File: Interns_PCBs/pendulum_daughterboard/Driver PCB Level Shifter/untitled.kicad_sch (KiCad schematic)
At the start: 10 parts, among them U5 AMS1117-3.3, U6 SN74LVC2T45DCUR

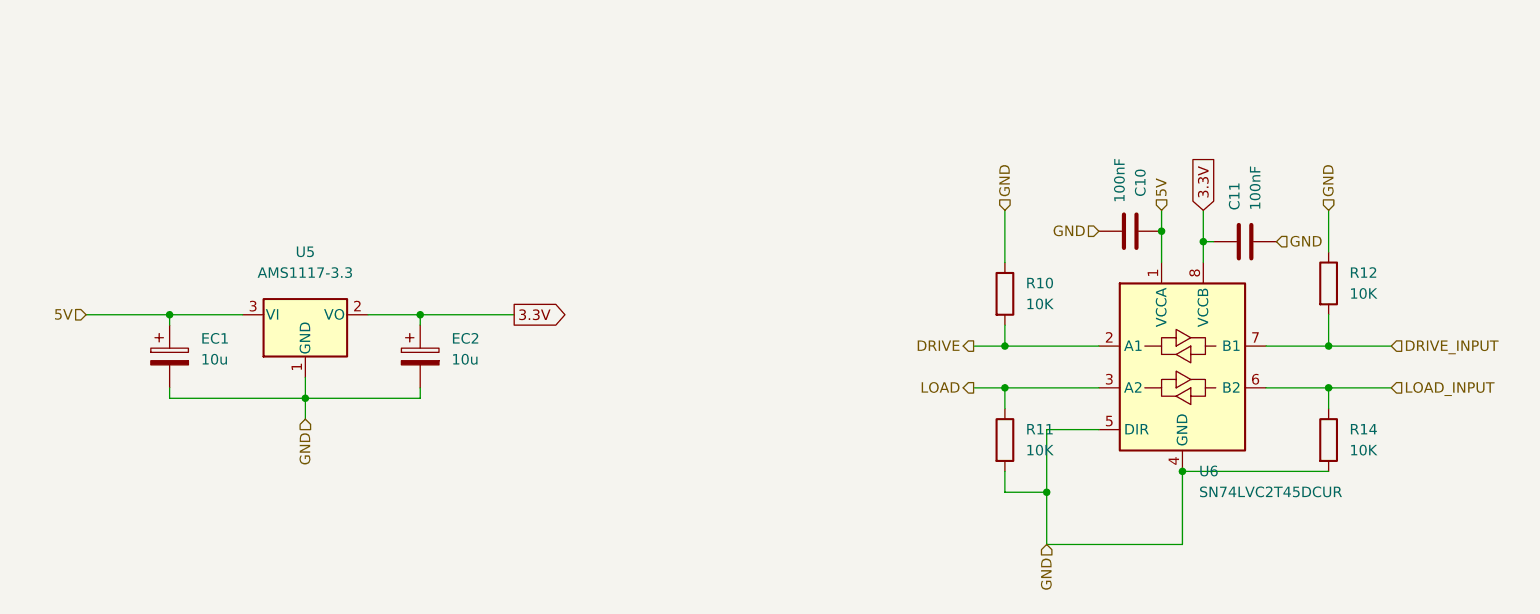
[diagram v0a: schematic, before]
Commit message: new PCB design started
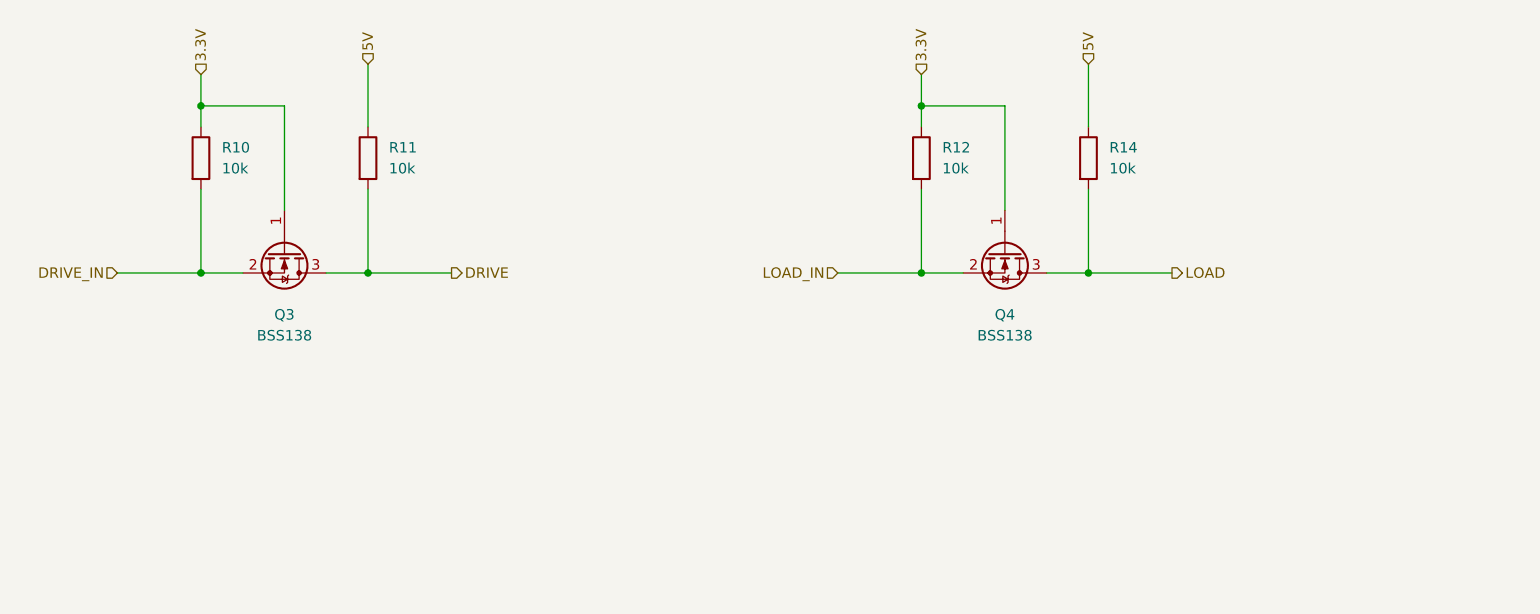
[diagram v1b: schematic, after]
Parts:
- removed C10, C11: 100nF, Capacitor_SMD:C_0805_2012Metric_Pad1.18x1.45mm_HandSolder, symbol Device:C
- removed EC1, EC2: 10u, Capacitor_SMD:CP_Elec_4x5.4, symbol 000_Capacitor_Electrolytic_Immo:22u
- removed U5: AMS1117-3.3, Package_TO_SOT_SMD:SOT-223-3_TabPin2, symbol Regulator_Linear:AMS1117-3.3
- removed U6: SN74LVC2T45DCUR, Package_SO:VSSOP-8_2.4x2.1mm_P0.5mm, symbol Logic_LevelTranslator:SN74LVC2T45DCUR
- added Q3, Q4: BSS138, Package_TO_SOT_SMD:SOT-23, symbol Transistor_FET:BSS138
- R10, R11, R12, R14: value 10K -> 10k; footprint Resistor_SMD:R_0805_2012Metric_Pad1.20x1.40mm_HandSolder -> (none)
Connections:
- net LOAD_INPUT is gone; now on net 5V: R14.1
- net 3.3V: now also R10.1, R12.1, Q3.1 (G), Q4.1 (G)
- net 5V: now also R11.1
- net DRIVE: now also R11.2, Q3.3 (D); no longer R10.2
- net LOAD: now also R14.2, Q4.3 (D); no longer R11.1
- net DRIVE_INPUT renamed LOAD_IN
- net LOAD_IN: now also Q4.2 (S)
- removed net GND: R10.1, R11.2, R12.1, R14.2
- new net DRIVE_IN: Q3.2 (S), R10.2

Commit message: Level Shifting Daughterboard
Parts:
- R10, R11, R12, R14: footprint (none) -> Resistor_SMD:R_0805_2012Metric_Pad1.20x1.40mm_HandSolder
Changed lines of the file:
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@@
       (effects (font (size 1.27 1.27)) (justify left))
     )
-    (property "Footprint" "" (id 2) (at 174.752 50.8 90)
+    (property "Footprint" "Resistor_SMD:R_0805_2012Metric_Pad1.20x1.40mm_HandSolder" (id 2) (at 174.752 50.8 90)
       (effects (font (size 1.27 1.27)) hide)
     )
@@
       (effects (font (size 1.27 1.27)) (justify left))
     )
-    (property "Footprint" "" (id 2) (at 107.442 50.8 90)
+    (property "Footprint" "Resistor_SMD:R_0805_2012Metric_Pad1.20x1.40mm_HandSolder" (id 2) (at 107.442 50.8 90)
       (effects (font (size 1.27 1.27)) hide)
     )
@@
       (effects (font (size 1.27 1.27)) (justify left))
     )
-    (property "Footprint" "" (id 2) (at 195.072 50.8 90)
+    (property "Footprint" "Resistor_SMD:R_0805_2012Metric_Pad1.20x1.40mm_HandSolder" (id 2) (at 195.072 50.8 90)
       (effects (font (size 1.27 1.27)) hide)
     )
@@
       (effects (font (size 1.27 1.27)) (justify left))
     )
-    (property "Footprint" "" (id 2) (at 87.122 50.8 90)
+    (property "Footprint" "Resistor_SMD:R_0805_2012Metric_Pad1.20x1.40mm_HandSolder" (id 2) (at 87.122 50.8 90)
       (effects (font (size 1.27 1.27)) hide)
     )
